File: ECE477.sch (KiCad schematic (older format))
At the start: 55 parts, among them IC1 LP3852EMP-3.3_NOPB, IC2 BQ29330DBT, J1 P7805-2000-S, J2 Conn_01x05_Male, J3 Conn_01x05_Male, J4 Conn_01x05_Male, J5 Conn_01x05_Male, J6 Conn_01x05_Male, SW1 SW_Push_Dual, U1 STM32H7_LQFP144_T2

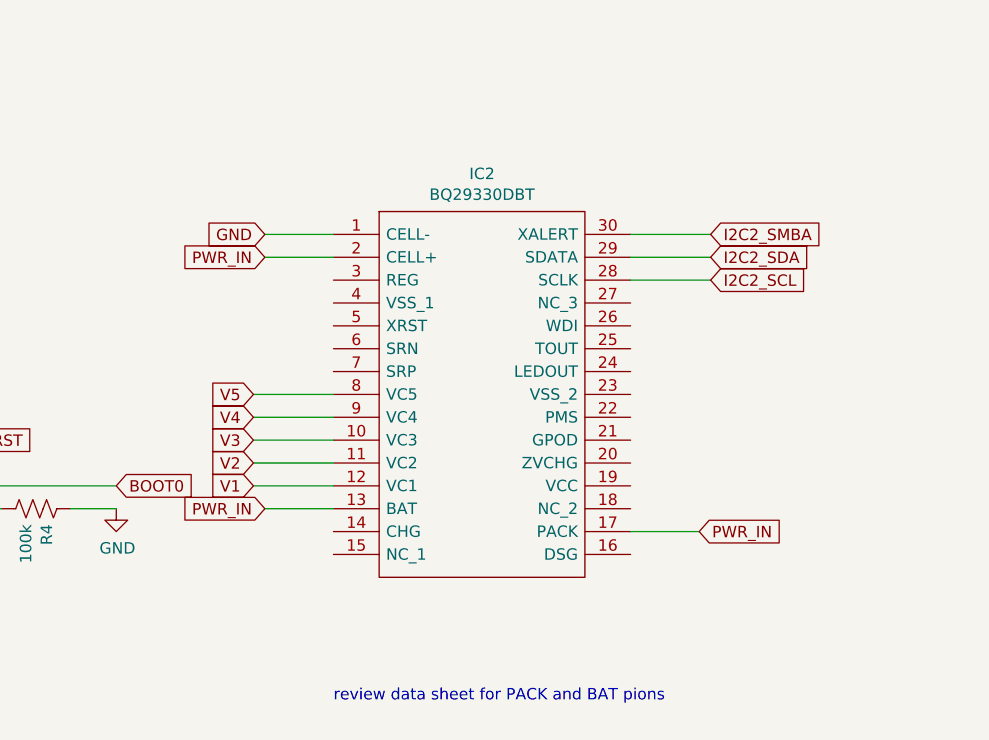
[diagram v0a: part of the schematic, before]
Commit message: Updated Bat monitor
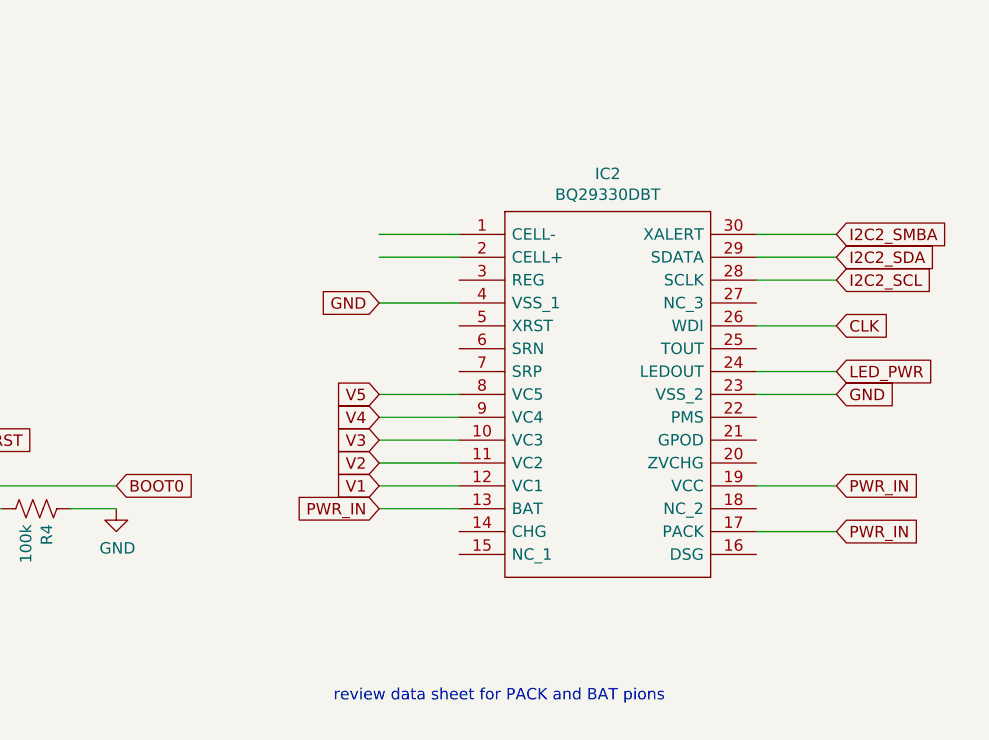
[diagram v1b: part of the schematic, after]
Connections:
- net GND: now also IC2.23 (VSS_2), IC2.4 (VSS_1); no longer IC2.1 (CELL-)
- net PWR_IN: now also IC2.19 (VCC); no longer IC2.2 (CELL+)
- net LED_PWR: now reaches IC2.24 (LEDOUT)
- net CLK: now reaches IC2.26 (WDI)
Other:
- moved on the sheet: IC2
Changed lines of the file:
@@
 Touch_Input
 Wire Wire Line
-	16100 2000 16450 2000
-Wire Wire Line
-	16100 2100 16450 2100
-Wire Wire Line
-	16100 2200 16450 2200
-Text GLabel 16450 2000 2    50   Input ~ 0
+	16650 2000 17000 2000
+Wire Wire Line
+	16650 2100 17000 2100
+Wire Wire Line
+	16650 2200 17000 2200
+Text GLabel 17000 2000 2    50   Input ~ 0
 I2C2_SMBA
-Text GLabel 16450 2100 2    50   Input ~ 0
+Text GLabel 17000 2100 2    50   Input ~ 0
 I2C2_SDA
-Text GLabel 16450 2200 2    50   Input ~ 0
+Text GLabel 17000 2200 2    50   Input ~ 0
 I2C2_SCL
 $Comp
 L ECE477-rescue:BQ29330DBT-SamacSys_Parts IC2
 U 1 1 5F7B6D95
-P 14800 2000
-F 0 "IC2" H 15450 2265 50  0000 C CNN
-F 1 "BQ29330DBT" H 15450 2174 50  0000 C CNN
-F 2 "SamacSys_Parts:SOP50P640X120-30N" H 25950 4500 50  0001 L CNN
-F 3 "http://www.ti.com/general/docs/suppproductinfo.tsp?distId=26&gotoUrl=http%3A%2F%2Fwww.ti.com%2Flit%2Fgpn%2Fbq29330" H 25950 4400 50  0001 L CNN
-F 4 "TEXAS INSTRUMENTS - BQ29330DBT. - Li-Ion Battery, Li-Pol Full Protector, 2/3/4 Series, I2C interface, 4.5 V to 28 V supply, TSSOP-30" H 25950 4300 50  0001 L CNN "Description"
-F 5 "1.2" H 25950 4200 50  0001 L CNN "Height"
-F 6 "595-BQ29330DBT" H 25950 4100 50  0001 L CNN "Mouser Part Number"
-F 7 "https://www.mouser.co.uk/ProductDetail/Texas-Instruments/BQ29330DBT?qs=YxwvVplHM%2FnxR6WOWVPfQQ%3D%3D" H 25950 4000 50  0001 L CNN "Mouser Price/Stock"
-F 8 "Texas Instruments" H 25950 3900 50  0001 L CNN "Manufacturer_Name"
-F 9 "BQ29330DBT" H 25950 3800 50  0001 L CNN "Manufacturer_Part_Number"
-	1    14800 2000
+P 15350 2000
+F 0 "IC2" H 16000 2265 50  0000 C CNN
+F 1 "BQ29330DBT" H 16000 2174 50  0000 C CNN
+F 2 "SamacSys_Parts:SOP50P640X120-30N" H 26500 4500 50  0001 L CNN
+F 3 "http://www.ti.com/general/docs/suppproductinfo.tsp?distId=26&gotoUrl=http%3A%2F%2Fwww.ti.com%2Flit%2Fgpn%2Fbq29330" H 26500 4400 50  0001 L CNN
+F 4 "TEXAS INSTRUMENTS - BQ29330DBT. - Li-Ion Battery, Li-Pol Full Protector, 2/3/4 Series, I2C interface, 4.5 V to 28 V supply, TSSOP-30" H 26500 4300 50  0001 L CNN "Description"
+F 5 "1.2" H 26500 4200 50  0001 L CNN "Height"
+F 6 "595-BQ29330DBT" H 26500 4100 50  0001 L CNN "Mouser Part Number"
+F 7 "https://www.mouser.co.uk/ProductDetail/Texas-Instruments/BQ29330DBT?qs=YxwvVplHM%2FnxR6WOWVPfQQ%3D%3D" H 26500 4000 50  0001 L CNN "Mouser Price/Stock"
+F 8 "Texas Instruments" H 26500 3900 50  0001 L CNN "Manufacturer_Name"
+F 9 "BQ29330DBT" H 26500 3800 50  0001 L CNN "Manufacturer_Part_Number"
+	1    15350 2000
 	1    0    0    -1
 $EndComp
@@
 Text GLabel 9700 3300 2    50   Input ~ 0
 PWM5
-Wire Wire Line
-	14800 2000 14500 2000
-Wire Wire Line
-	14800 2100 14500 2100
-Text GLabel 14500 2000 0    50   Input ~ 0
-GND
-Text GLabel 14500 2100 0    50   Input ~ 0
+Text GLabel 17000 3100 2    50   Input ~ 0
 PWR_IN
 Wire Wire Line
-	14800 3100 14450 3100
-Wire Wire Line
-	14800 3000 14450 3000
-Wire Wire Line
-	14800 2900 14450 2900
-Wire Wire Line
-	14800 2800 14450 2800
-Wire Wire Line
-	14800 2700 14450 2700
-Text GLabel 14450 2700 0    50   Input ~ 0
+	15350 3100 15000 3100
+Wire Wire Line
+	15350 3000 15000 3000
+Wire Wire Line
+	15350 2900 15000 2900
+Wire Wire Line
+	15350 2800 15000 2800
+Wire Wire Line
+	15350 2700 15000 2700
+Text GLabel 15000 2700 0    50   Input ~ 0
 V5
-Text GLabel 14450 2800 0    50   Input ~ 0
+Text GLabel 15000 2800 0    50   Input ~ 0
 V4
-Text GLabel 14450 2900 0    50   Input ~ 0
+Text GLabel 15000 2900 0    50   Input ~ 0
 V3
-Text GLabel 14450 3000 0    50   Input ~ 0
+Text GLabel 15000 3000 0    50   Input ~ 0
 V2
-Text GLabel 14450 3100 0    50   Input ~ 0
+Text GLabel 15000 3100 0    50   Input ~ 0
 V1
 Wire Notes Line
@@
 Text Notes 14800 4050 0    50   ~ 0
 review data sheet for PACK and BAT pions\n
-Wire Wire Line
-	16100 3300 16400 3300
-Text GLabel 16400 3300 2    50   Input ~ 0
+Text GLabel 17000 3300 2    50   Input ~ 0
 PWR_IN
-Wire Wire Line
-	14800 3200 14500 3200
-Text GLabel 14500 3200 0    50   Input ~ 0
+Text GLabel 15000 3200 0    50   Input ~ 0
 PWR_IN
+Wire Wire Line
+	15350 2300 15000 2300
+Wire Wire Line
+	16650 2700 17000 2700
+Wire Wire Line
+	15000 2100 15350 2100
+Wire Wire Line
+	15000 2000 15350 2000
+Text GLabel 15000 2300 0    50   Input ~ 0
+GND
+Text GLabel 17000 2700 2    50   Input ~ 0
+GND
+Wire Wire Line
+	16650 3100 17000 3100
+Wire Wire Line
+	16650 3300 17000 3300
+Wire Wire Line
+	15000 3200 15350 3200
+Wire Wire Line
+	16650 2600 17000 2600
+Text GLabel 17000 2600 2    50   Input ~ 0
+LED_PWR
+Wire Wire Line
+	16650 2400 17000 2400
+Text GLabel 17000 2400 2    50   Input ~ 0
+CLK
 $EndSCHEMATC
